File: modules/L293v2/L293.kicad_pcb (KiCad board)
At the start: 2 copper layers, 40.6 x 40.6 mm, 44 parts, among them J1 2, J10 11, J11 12, J12 13, J13 A0, J14 A1, J15 A2, J16 A3, J17 A4, J18 A5, J19 Vcc, J2 3, J20 Gnd, J21 Pwr, J22 M1, J23 M2, J24 Conn_01x01_Male, J25 Conn_01x01_Male, J3 4, J4 5, J5 6, J6 7, J7 8, J8 9, J9 10, Q1 IRLML5203, U1 74LS175, U5 L293D, U6 L4940

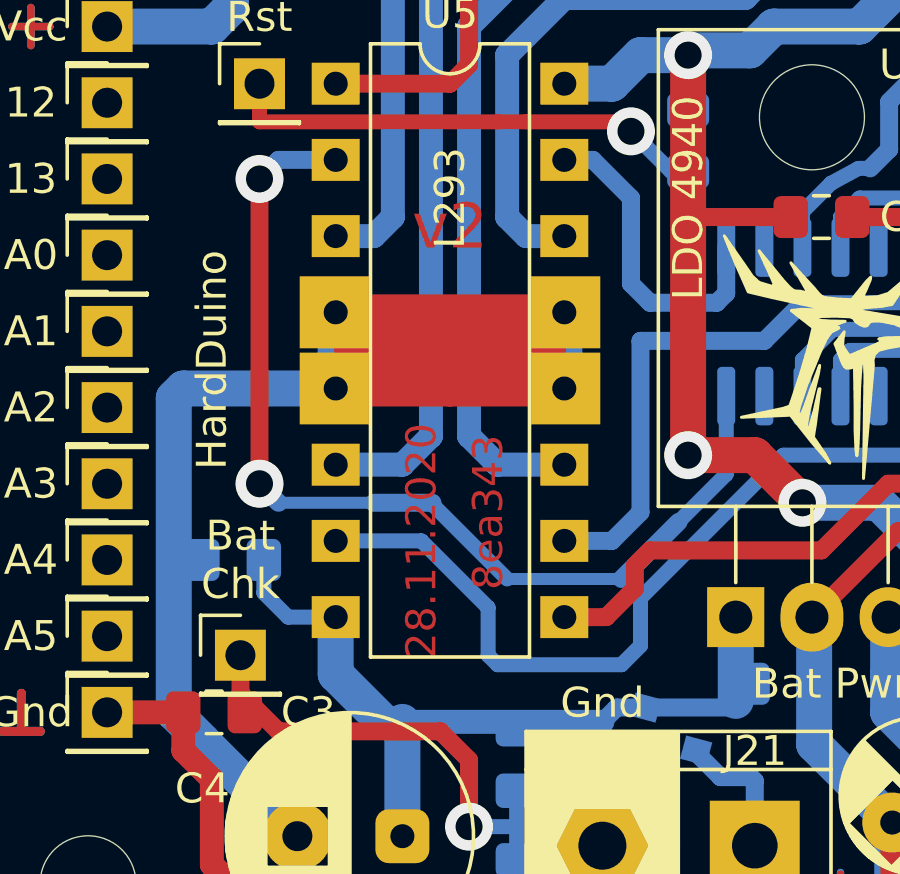
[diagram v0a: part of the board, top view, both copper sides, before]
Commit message: Fix hash & version
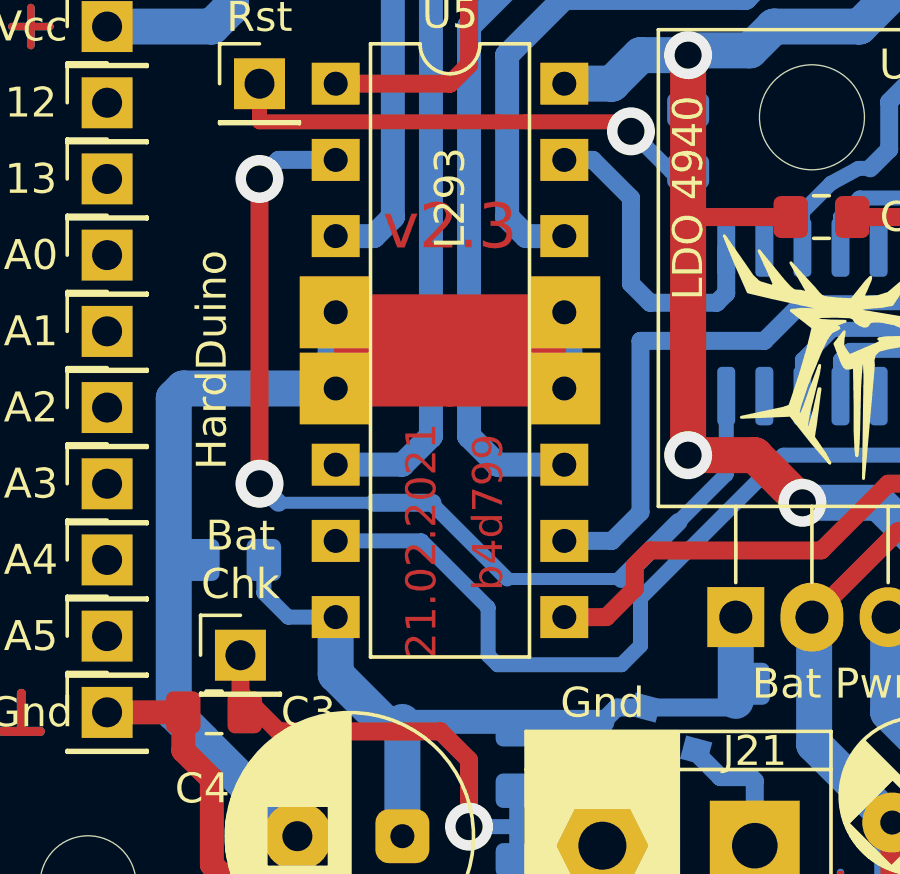
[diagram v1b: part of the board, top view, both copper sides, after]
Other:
- board text added: "21.02.2021"
- board text added: "b4d799"
- board text added: "v2.3"
- board text removed: "28.11.2020"
- board text removed: "8ea343"
- board text removed: "v2"
